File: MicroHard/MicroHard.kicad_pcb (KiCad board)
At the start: 6 copper layers, 198.2 x 104.1 mm, 193 parts, among them IC1 IS66WVO32M8DBLL-166BLI, J1 USB_B_Micro, J2 Micro_SD_Card_Det2, J3 GPIO_header, J4 MCU_Debug, J5 Controller Connector, J6 FPGA_GPIO_header, J7 FPGA_DEBUG, J8 L77HDE15SD1CH4FVGA, SW1 KMR221NGLFS, SW2 KMR221NGLFS, SW3 KMR221NGLFS, SW4 KMR221NGLFS, U1 TPS54325, U2 TPS54294, U3 EFM32GG842F1024, U4 XC7A100T-FTG256, U5 MAX6955 Display Driver, U6 SN74ALVC245PWR, U7 SN74ALVC245PWR, U8 MT25QL256ABA8ESF-0SIT, Y1 48MHz, Y2 CB3-3C-20M000000

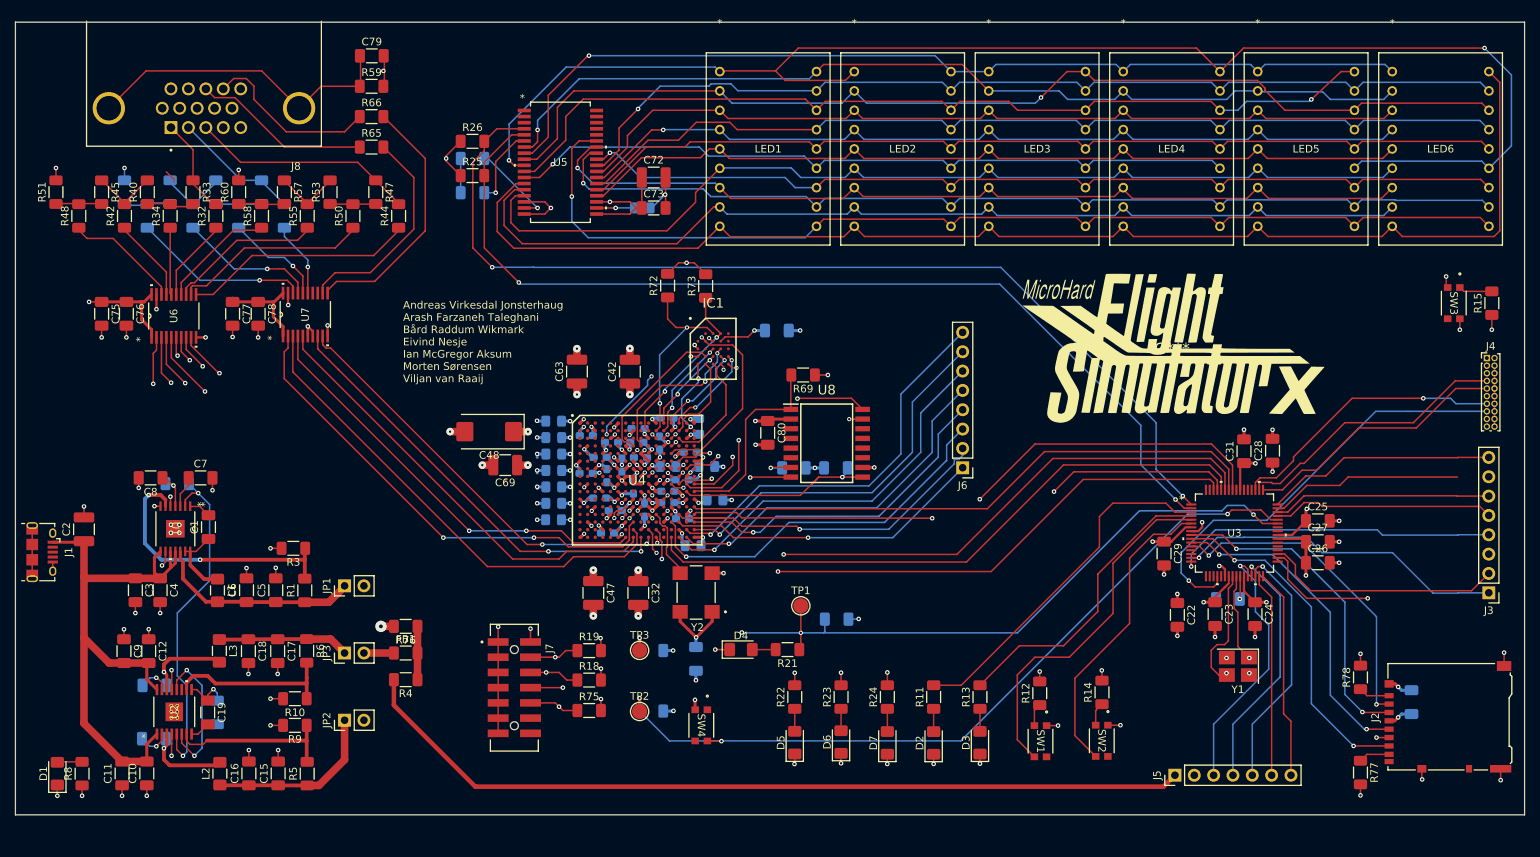
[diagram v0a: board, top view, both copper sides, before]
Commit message: Final changes
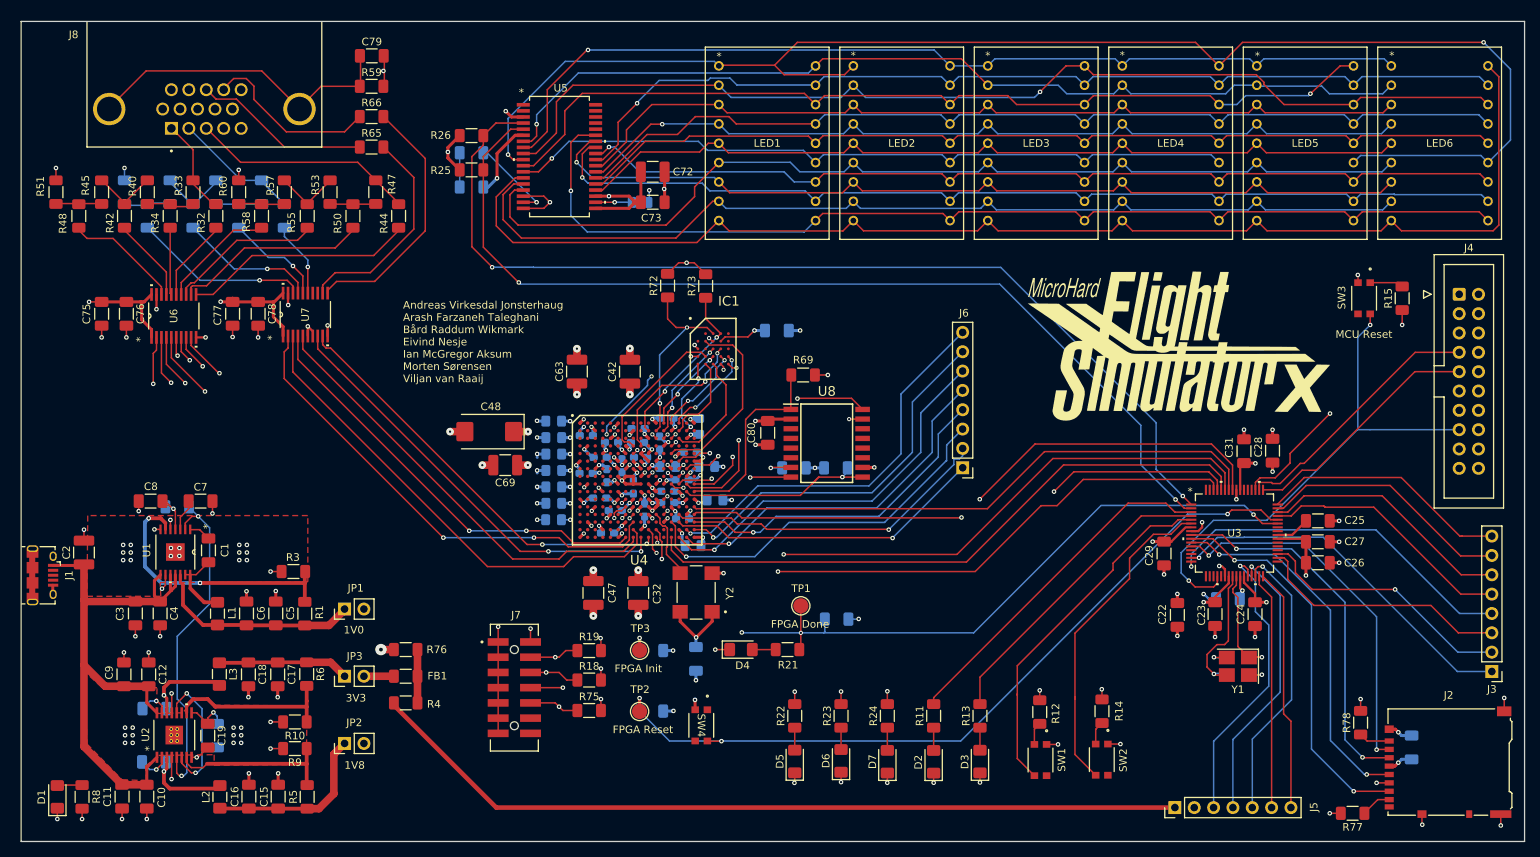
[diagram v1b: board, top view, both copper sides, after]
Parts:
- J4: footprint Connector_PinHeader_1.00mm:PinHeader_2x10_P1.00mm_Vertical -> Connector_IDC:IDC-Header_2x10_P2.54mm_Vertical
- moved R15 11.8 mm to (217.7, 77.9)
- moved SW3 11.8 mm to (212.7, 77.9)
- moved J3 10.3 mm to (229.5, 126.9)
- moved J4 9.13 mm to (225.2, 77.3)
- moved C82 5.95 mm to (219.0, 136.8)
- moved J2 5.95 mm to (223.8, 138.8)
- moved R78 5.95 mm to (212.3, 133.6)
- moved R77 5.45 mm to (211.2, 145.5), turned to 180 degrees
- moved J5 4.25 mm to (187.9, 144.8)
- moved C10 3.05 mm to (52.9, 143.3)
- moved C11 3.05 mm to (49.6, 143.3)
- moved C13 3.05 mm to (53.8, 138.8)
- moved C14 3.05 mm to (53.9, 131.8)
- moved C15 3.05 mm to (70.1, 143.3)
- moved C16 3.05 mm to (66.3, 143.3)
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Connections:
- U4 pad G10: GND -> +1V8
- U4 pad G8: GND -> +1V8
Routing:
- net Net-(J3-Pin_7): track 25.3 -> 33.2 mm
- net SD_US2_CLK: track 42.5 -> 48.7 mm
- net SD_US2_RX: track 44.7 -> 50.8 mm
- net SD_US2_CS: track 42.7 -> 48.7 mm
- net SD_US2_TX: track 42.7 -> 48.7 mm
- net Net-(U3B-PB14): track 12.0 -> 16.7 mm
- net US1_CS: track 43.0 -> 47.6 mm
- net US1_CLK: track 43.4 -> 48.1 mm
- net Net-(J6-Pin_2): track 49.0 -> 44.3 mm
- net Net-(J3-Pin_6): track 28.7 -> 33.3 mm
- net Net-(J3-Pin_5): track 29.2 -> 33.5 mm
- net Controller_Btn1: track 26.8 -> 31.1 mm
- net Controller_Z: track 33.1 -> 37.4 mm
- net Controller_X: track 34.1 -> 38.4 mm
- net Controller_Y: track 32.8 -> 37.0 mm
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- added copper zone on F.Cu, net GND
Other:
- board size 198.2 x 104.1 mm -> 197.5 x 107.7 mm
- board text added: "*"
